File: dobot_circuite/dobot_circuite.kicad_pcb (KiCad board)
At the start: 2 copper layers, 152 x 152 mm, 92 parts, among them J1 USB_A, J2 USB_A, J3 USB_A, J4 USB_A, J5 USB_A, J6 USB_A, J7 HDMI, J8 Jack-DC, J9 HDMI, K1 ALQ105, K2 ALQ105, K3 ALQ105, SW1 SW_Push_Dual, T1 2SD1781K, T2 2SD1781K, T3 2SD1781K, U1 FE1.1s, U10 fhoto_capura_PS817, U11 terminal_block_4pin_small, U12 fhoto_capura_PS817, U13 fhoto_capura_PS817, U14 fhoto_capura_PS817, U15 fhoto_capura_PS817, U16 terminal_block_4pin_small, U17 fhoto_capura_PS817, U18 fhoto_capura_PS817, U19 fhoto_capura_PS817, U2 microB_usb_connector, U20 diode_GS1010FL, U21 diode_GS1010FL, U22 diode_GS1010FL, U23 terminal_block_6pin_small, U3 microB_usb_connector, U5 microB_usb_connector, U7 HDMI_Hole2, U8 terminal_block_6pin_small, U9 terminal_block_2pin_small, Y1 Crystal

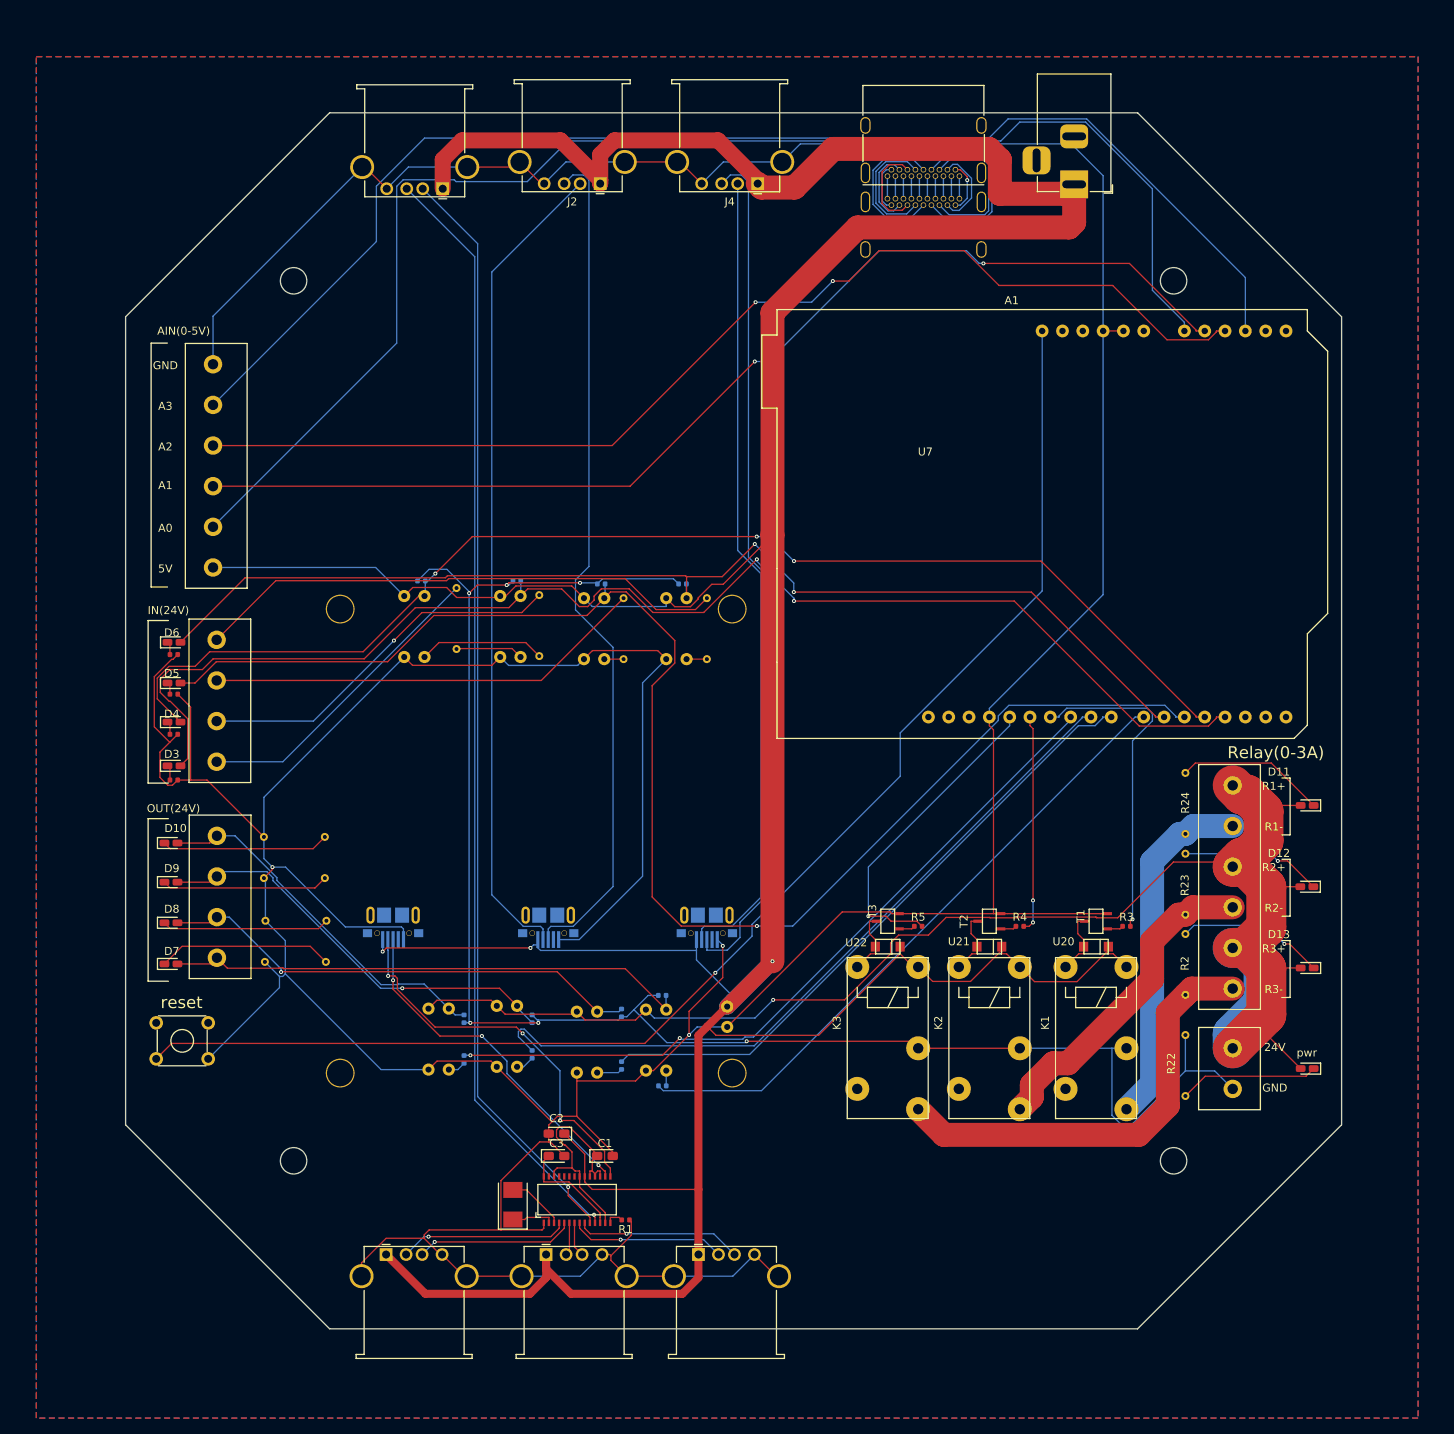
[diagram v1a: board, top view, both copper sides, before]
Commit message: Add files via upload
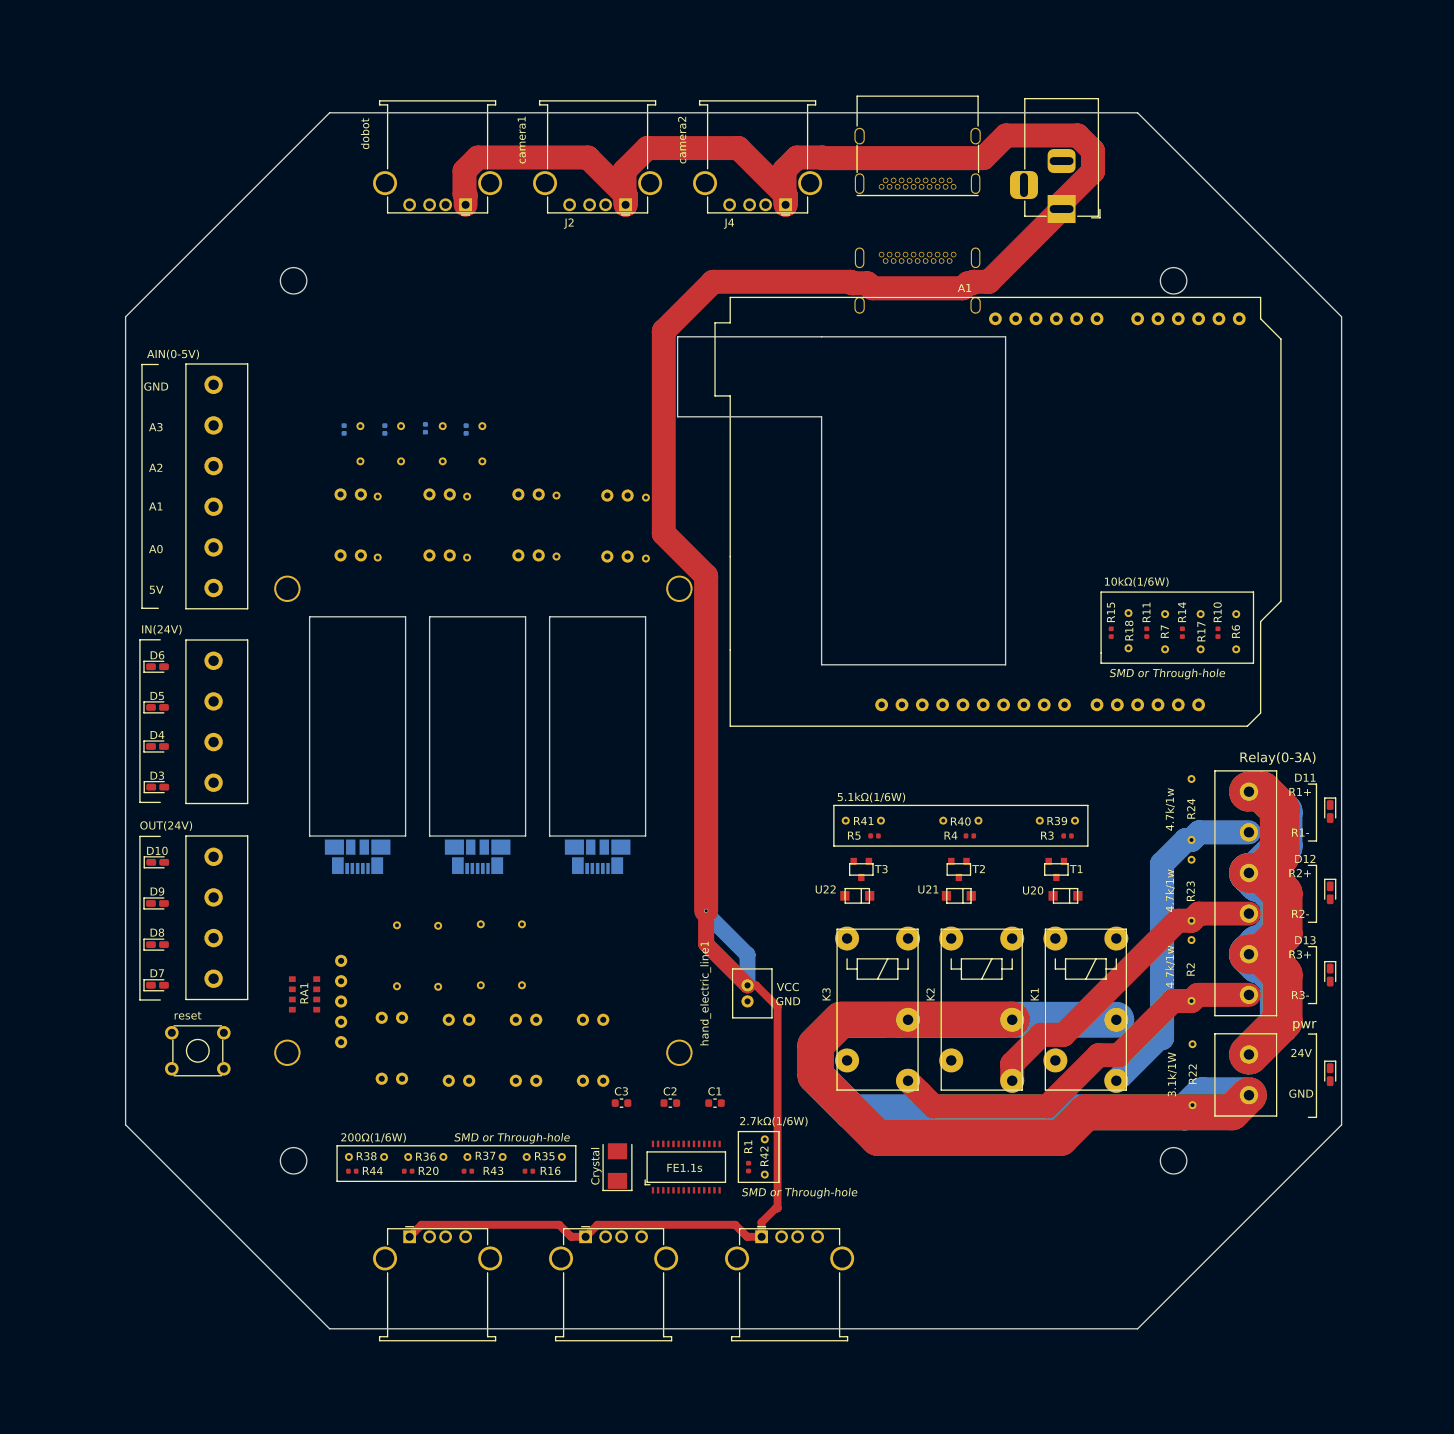
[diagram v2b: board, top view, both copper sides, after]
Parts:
- removed U2, U3, U5: microB_usb_connector, hoshina_library:USB_Micro-B_MC5F-03_aitendo_reverse
- removed U7: HDMI_Hole2, hoshina_library:HDMI_Hole2
- added J10: USB_B_Micro, hoshina_library:USB_Micro-B_Molex_47346-0001, B.Cu at (45.0, -60.0)
- added J11: USB_B_Micro, hoshina_library:USB_Micro-B_Molex_47346-0001, B.Cu at (60.0, -60.0)
- added J13: USB_B_Micro, hoshina_library:USB_Micro-B_Molex_47346-0001, B.Cu at (30.0, -60.0)
- added R33: R, hoshina_library:carbon_register_1_6W_, B.Cu at (40.6, -111.6)
- added R34: R, hoshina_library:carbon_register_1_6W_, B.Cu at (45.6, -111.6)
- added R35: R, hoshina_library:carbon_register_1_6W_, F.Cu at (53.3, -22.5)
- added R36: R, hoshina_library:carbon_register_1_6W_, F.Cu at (38.5, -22.5)
- added R37: R, hoshina_library:carbon_register_1_6W_, F.Cu at (45.9, -22.5)
- added R38: R, hoshina_library:carbon_register_1_6W_, F.Cu at (31.1, -22.5)
- added R39: R, hoshina_library:carbon_register_1_6W_, F.Cu at (117.5, -64.5)
- added R40: R, hoshina_library:carbon_register_1_6W_, F.Cu at (105.4, -64.5)
- added R41: R, hoshina_library:carbon_register_1_6W_, F.Cu at (93.2, -64.5)
- added R42: R, hoshina_library:carbon_register_1_6W_, F.Cu at (80.9, -22.5)
- added R43: 200/0.06W_chip, hoshina_library:register_0603, F.Cu at (43.8, -20.7)
- added R44: 200/0.06W_chip, hoshina_library:register_0603, F.Cu at (29.3, -20.7)
- added RA1: YC324J-10KCT-ND, hoshina_library:YC324J-10KCT-ND, F.Cu at (24.9, -40.9)
- added U4: aray_register_10k(1/8W), hoshina_library:array_register, B.Cu at (27.9, -36.8)
- A1: value Arduino_Leonardo_pin_remove_2pin -> Arduino_Leonardo_pin_remove_4pin; footprint hoshina_library:arduino_leonard_remove_2pin -> hoshina_library:arduino_leonard_remove_4pin
- C1, C2, C3: footprint hoshina_library:CP_EIA-2012-12_Kemet-R_Pad1.30x1.05mm_HandSolder -> hoshina_library:capa1608
- R1: value R -> 2.7k_chip
- R10, R11, R14, R15: value 10k -> 10k/0.0025W; moved to F.Cu
- R16, R20: value 190 -> 200/0.06W_chip; moved to F.Cu
- R17, R6: value 190 -> R; footprint hoshina_library:register_0603 -> hoshina_library:carbon_register_1_6W_; moved to F.Cu
- R18, R7: value 10k -> R; footprint hoshina_library:register_0603 -> hoshina_library:carbon_register_1_6W_; moved to F.Cu
- R19, R21: value 10k -> R; footprint hoshina_library:register_0603 -> hoshina_library:carbon_register_1_6W_
- R2, R23, R24, R29, R30, R31, R32: value 5.6k/1w -> 4.7k/1w
- R22: value R -> 3.1k/1W
- R25, R26, R27, R28: value 4.7k -> 4.7k/0.06W; moved to B.Cu
- R3, R4, R5: value 5k -> 5.1k/0.005W
- T1, T2, T3: value 2SD1781K -> S9013_trangister_elecrow; footprint hoshina_library:2SD1781 -> hoshina_library:S9013
- hand_electric_line1: footprint hoshina_library:2pin_power_gnd -> hoshina_library:XH2_pin
- moved J1 138.0 mm to (84.0, -12.5), turned to 0 degrees
- moved J3 131.4 mm to (40.0, -141.5), turned to 180 degrees
- moved R6 110.3 mm to (139.8, -88.1), turned to 270 degrees
- moved R7 100.1 mm to (130.9, -88.1), turned to 270 degrees
- moved R17 98.9 mm to (135.4, -88.1), turned to 270 degrees
- moved R14 95.3 mm to (133.1, -88.0), turned to 270 degrees
- moved R10 87.9 mm to (137.5, -88.0), turned to 270 degrees
- moved R21 78.3 mm to (30.4, -111.6), turned to 270 degrees
- moved R18 74.0 mm to (126.4, -88.3), turned to 270 degrees
- moved R19 73.7 mm to (35.4, -111.6)
- moved R11 68.5 mm to (128.7, -88.0), turned to 270 degrees
- moved R15 53.9 mm to (124.2, -88.0), turned to 270 degrees
- moved R26 48.7 mm to (28.3, -113.4), turned to 90 degrees
- moved R25 46.3 mm to (33.4, -113.4), turned to 90 degrees
- moved R28 46.1 mm to (43.6, -113.4), turned to 90 degrees
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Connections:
- R17 pad 1: Net-(R17-Pad1) -> GNDA
- R17 pad 2: D9 -> D4
- R18 pad 2: D7_24V -> D6
- R19 pad 1: GNDA -> GND
- R19 pad 2: D9_24V -> Net-(R19-Pad2)
- R20 pad 2: D8 -> D9
- R21 pad 1: GNDA -> GND
- R21 pad 2: D8_24V -> Net-(R21-Pad2)
- R25 pad 1: Net-(R25-Pad1) -> Net-(R19-Pad2)
- R26 pad 1: Net-(R26-Pad1) -> Net-(R21-Pad2)
- R6 pad 1: Net-(R6-Pad1) -> GNDA
- R6 pad 2: D10 -> D3
- R7 pad 2: D10_24V -> D5
- U10 pad 1: Net-(R6-Pad1) -> Net-(R38-Pad2)
- U18 pad 1: Net-(R17-Pad1) -> Net-(R20-Pad1)
- U19 pad 1: Net-(R20-Pad1) -> Net-(R37-Pad2)
- led4 pad 1: Net-(R25-Pad1) -> Net-(R19-Pad2)
- led5 pad 1: Net-(R26-Pad1) -> Net-(R21-Pad2)
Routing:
- net GND: track 698.6 -> 0.00 mm, vias 3 -> 0
- net +5V: track 549.2 -> 347.3 mm, vias 3 -> 1
- net D5: track 184.6 -> 0.00 mm, vias 1 -> 0
- net A0: track 172.9 -> 0.00 mm
- net Net-(A1-PadRESET): track 171.5 -> 0.00 mm, vias 1 -> 0
- net D3: track 168.0 -> 0.00 mm, vias 2 -> 0
- net A3: track 162.8 -> 0.00 mm
- net D4: track 155.4 -> 0.00 mm, vias 3 -> 0
- net D6: track 142.3 -> 0.00 mm, vias 2 -> 0
- net A2: track 141.7 -> 0.00 mm, vias 2 -> 0
- net A1: track 140.4 -> 0.00 mm, vias 2 -> 0
- net Net-(J1-Pad3): track 139.4 -> 0.00 mm, vias 1 -> 0
- net Net-(J1-Pad2): track 137.9 -> 0.00 mm, vias 1 -> 0
- net Net-(J11-Pad3): track 106.8 -> 0.00 mm
- net +24V: track 196.3 -> 89.8 mm, vias 1 -> 0
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- removed copper zone on B.Cu, net GND
- removed copper zone on F.Cu, net GND
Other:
- outline, holes or cut-outs redrawn
- board text added: "10kΩ(1/6W)"
- board text added: "2.7kΩ(1/6W)"
- board text added: "200Ω(1/6W)"
- board text added: "4.7kΩ(1/6W)"
- board text added: "5.1kΩ(1/6W)"
- board text added: "SMD or Through-hole"
- board text added: "VCC"
- board text added: "camera1"
- board text added: "camera2"
- board text added: "dobot"
